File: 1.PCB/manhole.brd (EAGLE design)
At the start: 66.3 x 76.5 mm, 23 parts, among them IC1 7805TV

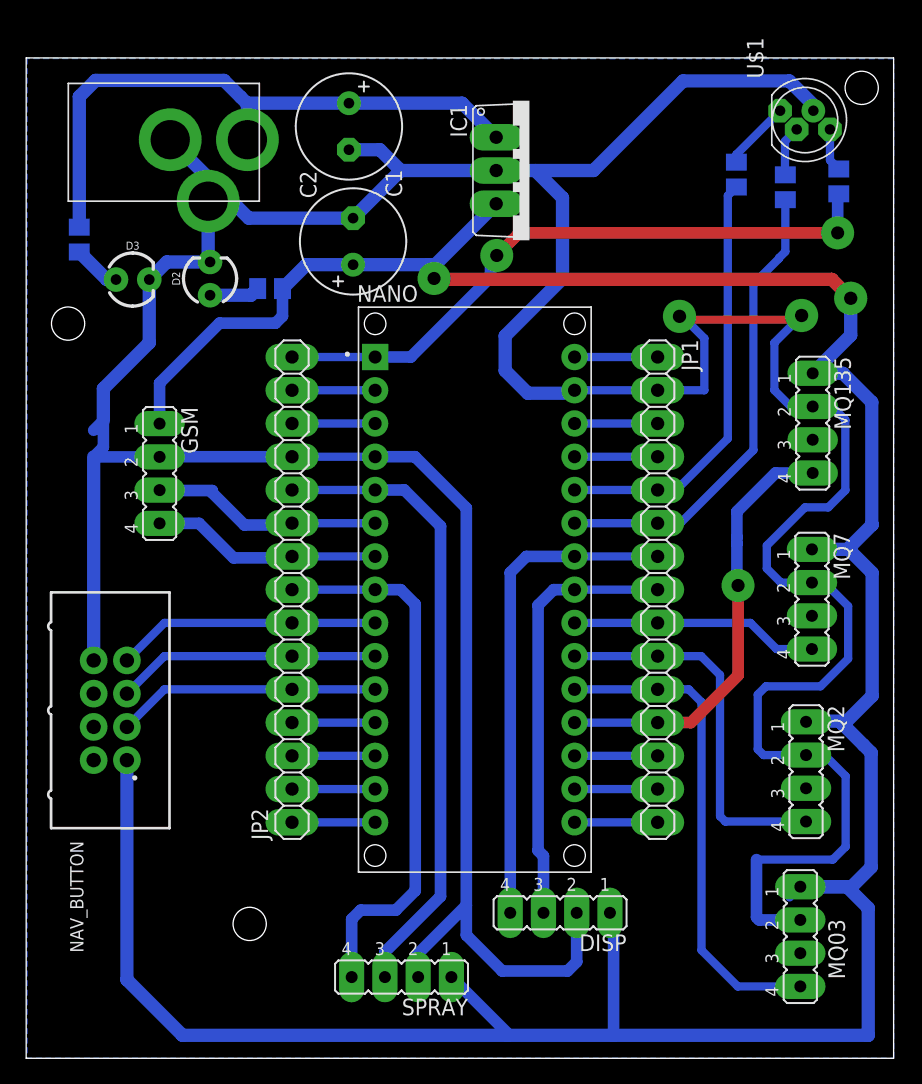
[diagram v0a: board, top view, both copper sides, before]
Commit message: updated PCB
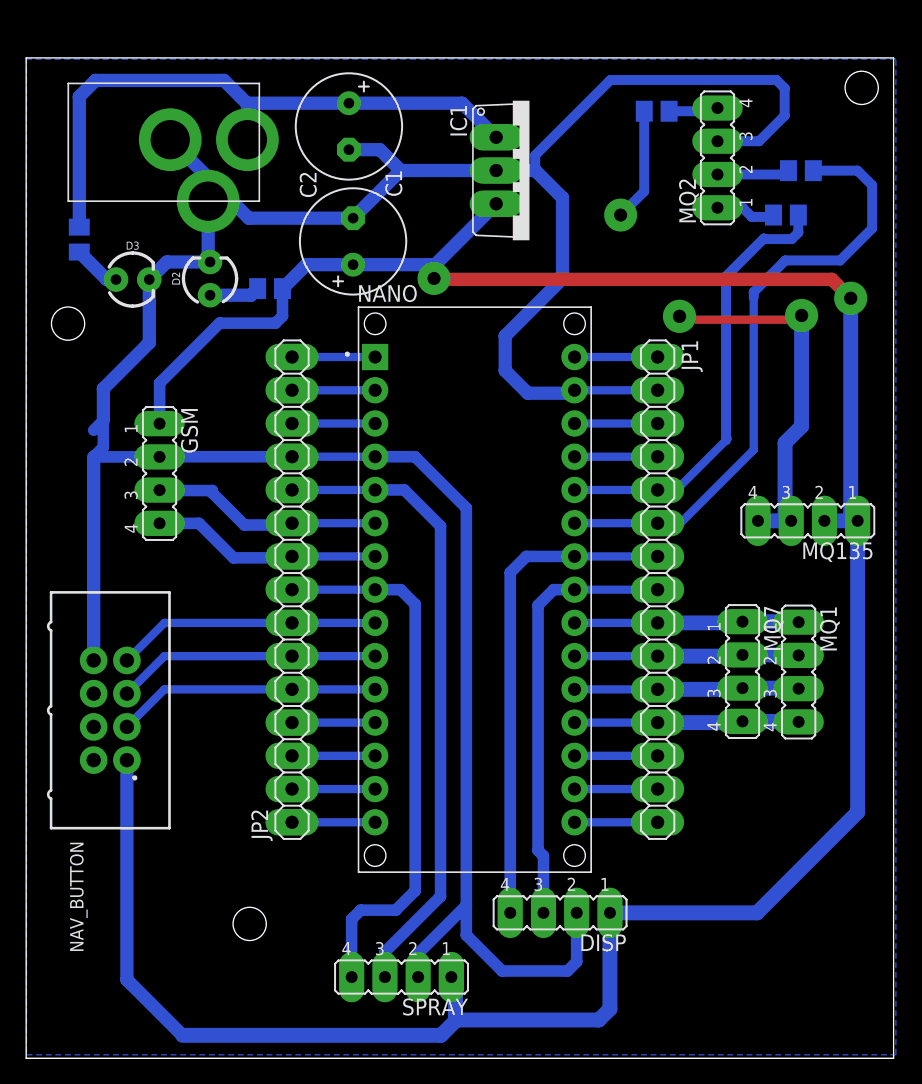
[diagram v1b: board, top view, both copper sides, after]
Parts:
- removed MQ03: (no value), jumper:JP4
- removed U$1: 5MMRGBLED, led_rgb:LED5MMRGB
- added MQ1: (no value), jumper:JP4
- moved MQ2 47.4 mm to (52.8, 68.6), turned to 90 degrees
- moved R1 14.9 mm to (48.2, 72.1), turned to 0 degrees
- moved MQ7 7.66 mm to (54.7, 29.3)
- moved MQ135 7.48 mm to (59.7, 40.8), turned to 180 degrees
- moved R3 4.89 mm to (58.1, 64.2), turned to 180 degrees
- moved R2 1.74 mm to (59.2, 67.6), turned to 180 degrees
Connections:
- removed net MQ135D0: MQ135.3
- removed net MQ2D0: MQ2.3
- removed net MQ3A0: JP1.11, MQ03.4, NANO.20
- removed net MQ3D0: MQ03.3
- removed net MQ7D0: MQ7.3
- removed net SS: JP2.3, NANO.13
- new net D0: JP2.15, NANO.1
- new net MQ6A0: JP1.10, MQ1.2, MQ7.2, NANO.21
- net 5V: now also MQ135.2; no longer MQ03.1, MQ2.1, MQ7.1
- net BLUE: now also MQ2.1; no longer U$1.P$1
- net GND: now also MQ135.3, MQ135.4, MQ2.3; no longer MQ03.2, MQ135.2, MQ2.2, MQ7.2, U$1.P$3
- net GREEN: now also MQ2.2; no longer U$1.P$2
- net MQ135A0: now also MQ1.4, MQ7.4; no longer MQ135.4
- net MQ2A0: now also JP1.9, MQ1.1, MQ7.1, NANO.22; no longer JP1.10, MQ2.4, NANO.21
- net MQ7A0: now also JP1.11, MQ1.3, MQ7.3, NANO.20; no longer JP1.9, MQ7.4, NANO.22
- net RED: now also MQ2.4; no longer U$1.P$4
- net RED1: now also JP2.3, NANO.13; no longer JP2.15, NANO.1
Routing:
- net GND: track 318.4 -> 253.6 mm
- net 5V: track 244.6 -> 202.0 mm
- net MQ3A0: track 37.8 -> 0.00 mm
- net RED1: track 49.4 -> 15.0 mm, vias 2 -> 1
- net MQ6A0: track 0.00 -> 17.2 mm
- net MQ135A0: track 33.6 -> 17.2 mm, vias 1 -> 0
- net MQ2A0: track 29.3 -> 17.2 mm
- net GREEN1: track 36.1 -> 47.4 mm
- net SS: track 6.35 -> 0.00 mm
- net D0: track 0.00 -> 6.35 mm
- net MQ7A0: track 19.0 -> 17.2 mm
- net GREEN: track 3.85 -> 5.54 mm
- net BLUE1: track 32.8 -> 34.2 mm
- net BLUE: track 5.32 -> 4.63 mm

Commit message: Revert "updated PCB"
This reverts commit e032bd37680646525048ee8d74092bea044d5abf.
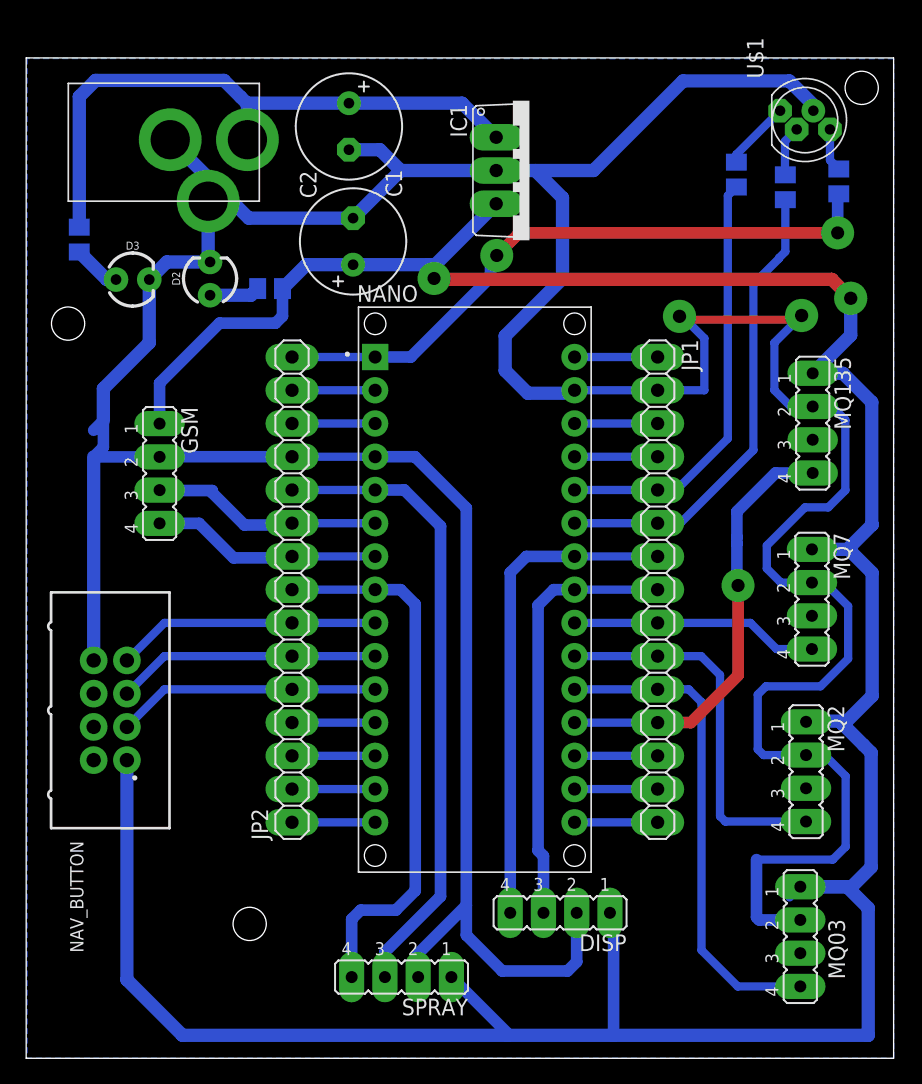
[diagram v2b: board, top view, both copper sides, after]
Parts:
- removed MQ1: (no value), jumper:JP4
- added MQ03: (no value), jumper:JP4
- added U$1: 5MMRGBLED, led_rgb:LED5MMRGB
- moved MQ2 47.4 mm to (59.6, 21.6), turned to 270 degrees
- moved R1 14.9 mm to (62.1, 66.8), turned to 270 degrees
- moved MQ7 7.66 mm to (60.1, 34.8)
- moved MQ135 7.48 mm to (60.1, 48.3), turned to 270 degrees
- moved R3 4.89 mm to (54.3, 67.3), turned to 270 degrees
- moved R2 1.74 mm to (58.0, 66.3), turned to 270 degrees
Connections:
- removed net D0: JP2.15, NANO.1
- removed net MQ6A0: JP1.10, MQ1.2, MQ7.2, NANO.21
- new net MQ135D0: MQ135.3
- new net MQ2D0: MQ2.3
- new net MQ3A0: JP1.11, MQ03.4, NANO.20
- new net MQ3D0: MQ03.3
- new net MQ7D0: MQ7.3
- new net SS: JP2.3, NANO.13
- net 5V: now also MQ03.1, MQ2.1, MQ7.1; no longer MQ135.2
- net BLUE: now also U$1.P$1; no longer MQ2.1
- net GND: now also MQ03.2, MQ135.2, MQ2.2, MQ7.2, U$1.P$3; no longer MQ135.3, MQ135.4, MQ2.3
- net GREEN: now also U$1.P$2; no longer MQ2.2
- net MQ135A0: now also MQ135.4; no longer MQ1.4, MQ7.4
- net MQ2A0: now also JP1.10, MQ2.4, NANO.21; no longer JP1.9, MQ1.1, MQ7.1, NANO.22
- net MQ7A0: now also JP1.9, MQ7.4, NANO.22; no longer JP1.11, MQ1.3, MQ7.3, NANO.20
- net RED: now also U$1.P$4; no longer MQ2.4
- net RED1: now also JP2.15, NANO.1; no longer JP2.3, NANO.13
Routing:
- net GND: track 253.6 -> 318.4 mm
- net 5V: track 202.0 -> 244.6 mm
- net MQ3A0: track 0.00 -> 37.8 mm
- net RED1: track 15.0 -> 49.4 mm, vias 1 -> 2
- net MQ6A0: track 17.2 -> 0.00 mm
- net MQ135A0: track 17.2 -> 33.6 mm, vias 0 -> 1
- net MQ2A0: track 17.2 -> 29.3 mm
- net GREEN1: track 47.4 -> 36.1 mm
- net SS: track 0.00 -> 6.35 mm
- net D0: track 6.35 -> 0.00 mm
- net MQ7A0: track 17.2 -> 19.0 mm
- net GREEN: track 5.54 -> 3.85 mm
- net BLUE1: track 34.2 -> 32.8 mm
- net BLUE: track 4.63 -> 5.32 mm
